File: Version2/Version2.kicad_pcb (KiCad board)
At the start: 4 copper layers, 50.8 x 87 mm, 134 parts, among them J1 USB_C_Receptacle_USB2.0_16P, J10 Conn_01x03, J11 Conn_01x03, J12 MSD-4-A, J13 Conn_01x04_Socket, J14 Conn_01x03, J15 Conn_01x03, J16 Conn_01x03, J17 Conn_01x03, J18 Conn_01x04_Socket, J19 Conn_01x04_Socket, J26 Conn_01x04_Socket, J27 Conn_01x02_Socket, J29 Conn_01x02_Socket, J30 Conn_01x02_Socket, J31 Conn_01x02_Socket, J5 Conn_01x02_Pin, J6 Conn_01x04_Socket, J7 Conn_01x03, J8 Conn_01x03, J9 Conn_01x04_Socket, SW1 SW_Push, SW2 SW_Push, U1 W25Q128JVS, U10 INA219AxDCN, U11 AP2112K-3.3, U12 AP62150WU, U13 TPS2121RUXR, U14 AP62150WU, U15 74AHC541, U2 RP2350B-QFN80, U3 MMC5983MA, U4 ICM-45686, U5 MS5611-01BA, U6 TMP117xxDRV, U8 KX134-1211, U9 TPS2121RUXR, Y1 ABM8-272-T3

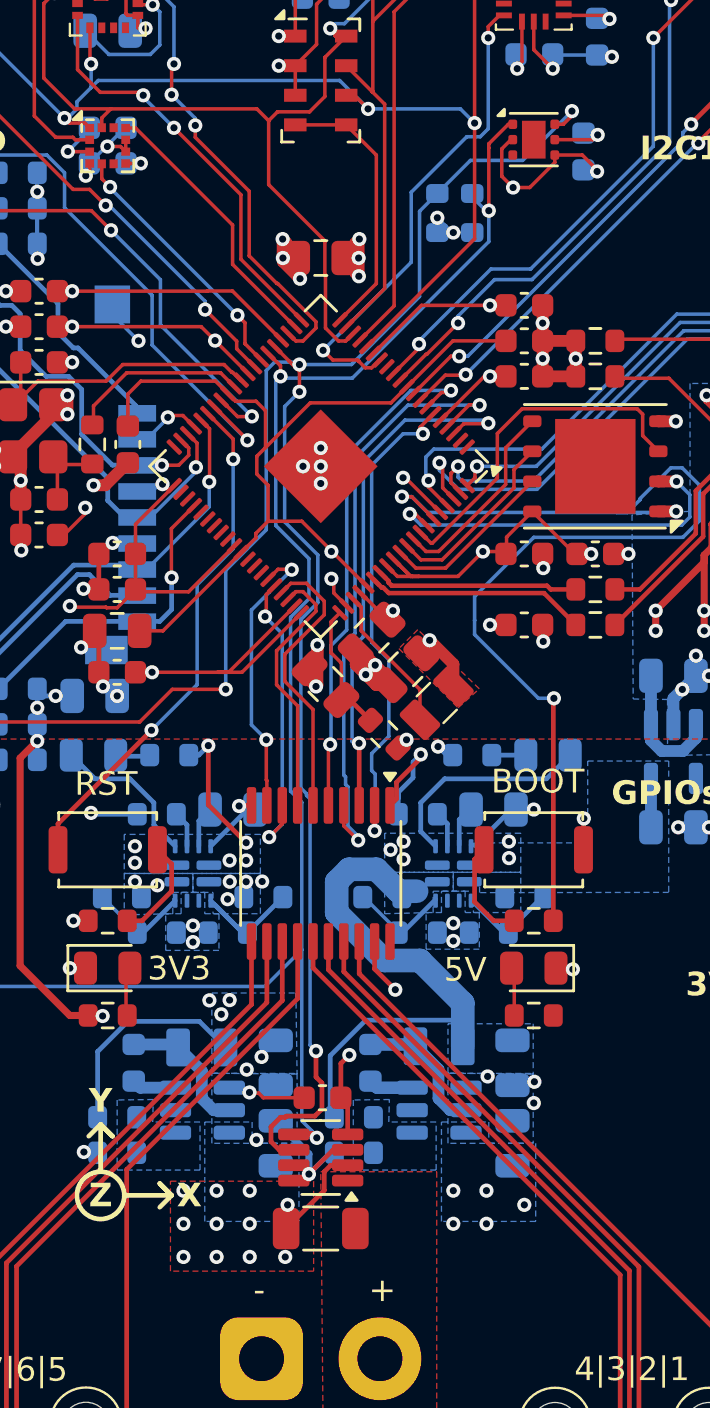
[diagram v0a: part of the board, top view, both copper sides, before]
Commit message: Small Fixes
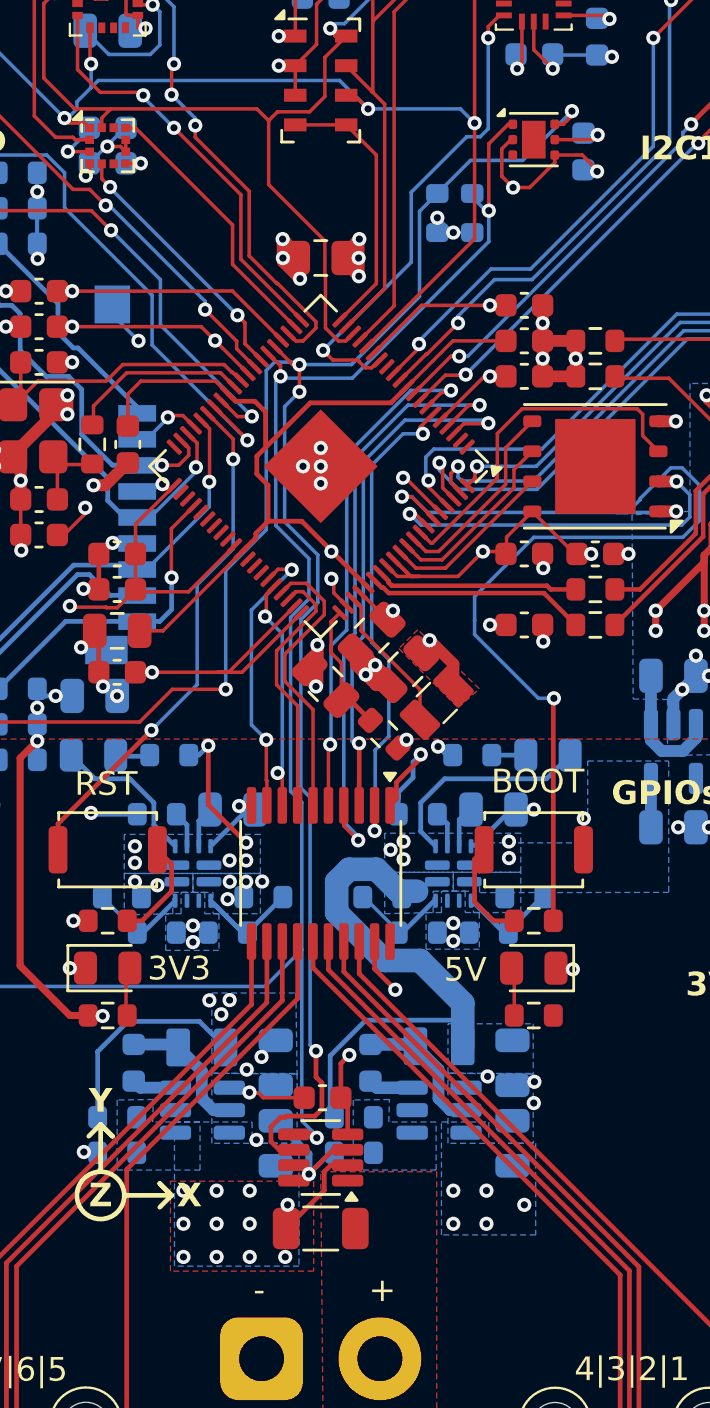
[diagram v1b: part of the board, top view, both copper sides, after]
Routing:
- net PWM7: track 12.9 -> 9.90 mm
- removed copper zone on In2.Cu, net +5V
